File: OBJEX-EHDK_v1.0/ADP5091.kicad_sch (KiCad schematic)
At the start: 33 parts, among them J15 Solar, J16 Vout1, J17 Vout2, J18 Conn_01x02, J19 Conn_01x02, J20 TestPoint - Black, J21 TestPoint - Red, J22 TestPoint - Purple, J23 TestPoint - Orange, J24 TestPoint - Black, J25 TestPoint - Black, U2 ADP5091

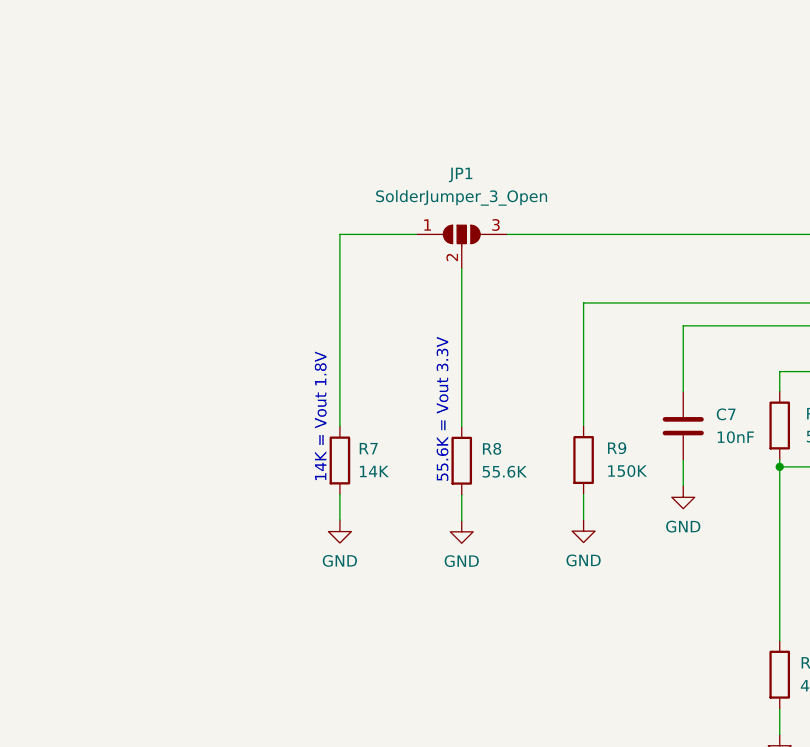
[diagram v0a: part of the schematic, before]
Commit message: SCH first review
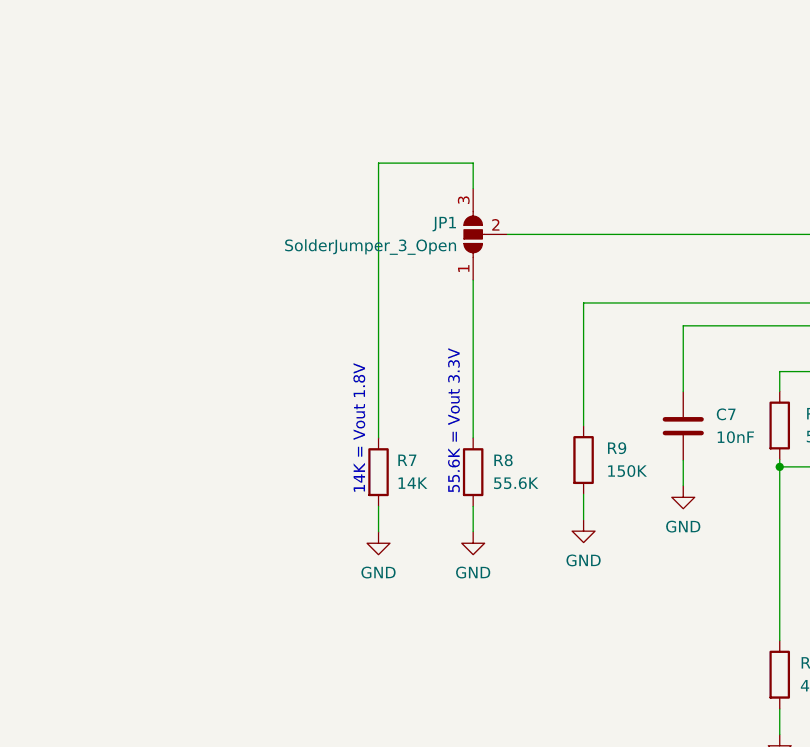
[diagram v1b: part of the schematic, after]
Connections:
- net at U2.20 (VID): now also JP1.2 (C); no longer JP1.3 (B)
- net at R8.1: now also JP1.1 (A); no longer JP1.2 (C)
- net at R7.1: now also JP1.3 (B); no longer JP1.1 (A)
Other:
- moved on the sheet: JP1, R7, R8
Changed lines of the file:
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@@
+    (stroke (width 0) (type default) (color 0 0 0 0))
+  )
+  (wire (pts (xy 69.0626 85.2678) (xy 69.0626 88.1126))
     (stroke (width 0) (type default) (color 0 0 0 0))
   )
@@
     (stroke (width 0) (type default) (color 0 0 0 0))
   )
+  (wire (pts (xy 58.547 85.2678) (xy 69.0626 85.2678))
+    (stroke (width 0) (type default) (color 0 0 0 0))
+  )
   (wire (pts (xy 137.6426 76.0222) (xy 137.6426 77.9526))
     (stroke (width 0) (type default) (color 0 0 0 0))
@@
     (stroke (width 0) (type default) (color 0 0 0 0))
   )
-  (wire (pts (xy 54.2544 93.1926) (xy 54.2544 114.5032))
+  (wire (pts (xy 58.547 85.2678) (xy 58.547 115.7986))
     (stroke (width 0) (type default) (color 0 0 0 0))
   )
@@
     (stroke (width 0) (type default) (color 0 0 0 0))
   )
-  (wire (pts (xy 67.7926 114.5286) (xy 67.7926 97.0026))
+  (wire (pts (xy 69.0626 115.7986) (xy 69.0626 98.2726))
     (stroke (width 0) (type default) (color 0 0 0 0))
   )
@@
     (stroke (width 0) (type default) (color 0 0 0 0))
   )
-  (wire (pts (xy 62.7126 93.1926) (xy 54.2544 93.1926))
-    (stroke (width 0) (type default) (color 0 0 0 0))
-  )
   (wire (pts (xy 212.217 103.3526) (xy 212.217 105.664))
     (stroke (width 0) (type default) (color 0 0 0 0))
@@
     (stroke (width 0) (type default) (color 0 0 0 0))
   )
-  (wire (pts (xy 54.2544 122.1232) (xy 54.2544 124.9426))
+  (wire (pts (xy 58.547 123.4186) (xy 58.547 126.238))
     (stroke (width 0) (type default) (color 0 0 0 0))
   )
@@
     (stroke (width 0) (type default) (color 0 0 0 0))
   )
-  (wire (pts (xy 67.7926 122.1486) (xy 67.7926 124.968))
+  (wire (pts (xy 69.0626 123.4186) (xy 69.0626 126.238))
     (stroke (width 0) (type default) (color 0 0 0 0))
   )
@@
     (effects (font (size 5 5) (thickness 0.8) bold) (justify left bottom))
   )
-  (text "55.6K = Vout 3.3V" (at 66.4464 120.9548 90)
+  (text "55.6K = Vout 3.3V" (at 67.7164 122.2248 90)
     (effects (font (size 1.27 1.27)) (justify left bottom))
   )
@@
     (effects (font (size 3.5 3.5) italic) (justify left bottom))
   )
-  (text "14K = Vout 1.8V" (at 52.9082 120.9294 90)
+  (text "14K = Vout 1.8V" (at 57.2008 122.2248 90)
     (effects (font (size 1.27 1.27)) (justify left bottom))
   )
@@
     (pin "2")
   )
-  (symbol (lib_id "power:GND") (at 54.2544 124.9426 0) (unit 1)
-    (in_bom yes) (on_board yes) (fields_autoplaced)
-    (property "Reference" "#PWR0125" (id 0) (at 54.2544 131.2926 0)
-      (effects (font (size 1.27 1.27)) hide)
-    )
-    (property "Value" "GND" (id 1) (at 54.2544 129.5146 0))
-    (property "Footprint" "" (id 2) (at 54.2544 124.9426 0)
-      (effects (font (size 1.27 1.27)) hide)
-    )
-    (property "Datasheet" "" (id 3) (at 54.2544 124.9426 0)
+  (symbol (lib_id "power:GND") (at 58.547 126.238 0) (unit 1)
+    (in_bom yes) (on_board yes) (fields_autoplaced)
+    (property "Reference" "#PWR0125" (id 0) (at 58.547 132.588 0)
+      (effects (font (size 1.27 1.27)) hide)
+    )
+    (property "Value" "GND" (id 1) (at 58.547 130.81 0))
+    (property "Footprint" "" (id 2) (at 58.547 126.238 0)
+      (effects (font (size 1.27 1.27)) hide)
+    )
+    (property "Datasheet" "" (id 3) (at 58.547 126.238 0)
       (effects (font (size 1.27 1.27)) hide)
     )
@@
     (pin "2")
   )
-  (symbol (lib_id "power:GND") (at 67.7926 124.968 0) (unit 1)
-    (in_bom yes) (on_board yes) (fields_autoplaced)
-    (property "Reference" "#PWR0124" (id 0) (at 67.7926 131.318 0)
-      (effects (font (size 1.27 1.27)) hide)
-    )
-    (property "Value" "GND" (id 1) (at 67.7926 129.54 0))
-    (property "Footprint" "" (id 2) (at 67.7926 124.968 0)
-      (effects (font (size 1.27 1.27)) hide)
-    )
-    (property "Datasheet" "" (id 3) (at 67.7926 124.968 0)
+  (symbol (lib_id "power:GND") (at 69.0626 126.238 0) (unit 1)
+    (in_bom yes) (on_board yes) (fields_autoplaced)
+    (property "Reference" "#PWR0124" (id 0) (at 69.0626 132.588 0)
+      (effects (font (size 1.27 1.27)) hide)
+    )
+    (property "Value" "GND" (id 1) (at 69.0626 130.81 0))
+    (property "Footprint" "" (id 2) (at 69.0626 126.238 0)
+      (effects (font (size 1.27 1.27)) hide)
+    )
+    (property "Datasheet" "" (id 3) (at 69.0626 126.238 0)
       (effects (font (size 1.27 1.27)) hide)
     )
@@
     (pin "1")
   )
-  (symbol (lib_id "Device:R") (at 67.7926 118.3386 0) (unit 1)
-    (in_bom yes) (on_board yes) (fields_autoplaced)
-    (property "Reference" "R8" (id 0) (at 69.977 117.0685 0)
-      (effects (font (size 1.27 1.27)) (justify left))
-    )
-    (property "Value" "55.6K" (id 1) (at 69.977 119.6085 0)
-      (effects (font (size 1.27 1.27)) (justify left))
-    )
-    (property "Footprint" "Resistor_SMD:R_0603_1608Metric" (id 2) (at 66.0146 118.3386 90)
-      (effects (font (size 1.27 1.27)) hide)
-    )
-    (property "Datasheet" "~" (id 3) (at 67.7926 118.3386 0)
+  (symbol (lib_id "Device:R") (at 69.0626 119.6086 0) (unit 1)
+    (in_bom yes) (on_board yes) (fields_autoplaced)
+    (property "Reference" "R8" (id 0) (at 71.247 118.3385 0)
+      (effects (font (size 1.27 1.27)) (justify left))
+    )
+    (property "Value" "55.6K" (id 1) (at 71.247 120.8785 0)
+      (effects (font (size 1.27 1.27)) (justify left))
+    )
+    (property "Footprint" "Resistor_SMD:R_0603_1608Metric" (id 2) (at 67.2846 119.6086 90)
+      (effects (font (size 1.27 1.27)) hide)
+    )
+    (property "Datasheet" "~" (id 3) (at 69.0626 119.6086 0)
       (effects (font (size 1.27 1.27)) hide)
     )
@@
     (pin "2")
   )
-  (symbol (lib_id "Jumper:SolderJumper_3_Open") (at 67.7926 93.1926 0) (unit 1)
-    (in_bom yes) (on_board yes) (fields_autoplaced)
-    (property "Reference" "JP1" (id 0) (at 67.7926 86.4616 0))
-    (property "Value" "SolderJumper_3_Open" (id 1) (at 67.7926 89.0016 0))
-    (property "Footprint" "Jumper:SolderJumper-3_P1.3mm_Open_Pad1.0x1.5mm_NumberLabels" (id 2) (at 67.7926 93.1926 0)
-      (effects (font (size 1.27 1.27)) hide)
-    )
-    (property "Datasheet" "~" (id 3) (at 67.7926 93.1926 0)
+  (symbol (lib_id "Jumper:SolderJumper_3_Open") (at 69.0626 93.1926 90) (unit 1)
+    (in_bom yes) (on_board yes) (fields_autoplaced)
+    (property "Reference" "JP1" (id 0) (at 67.31 91.9225 90)
+      (effects (font (size 1.27 1.27)) (justify left))
+    )
+    (property "Value" "SolderJumper_3_Open" (id 1) (at 67.31 94.4625 90)
+      (effects (font (size 1.27 1.27)) (justify left))
+    )
+    (property "Footprint" "Jumper:SolderJumper-3_P1.3mm_Open_Pad1.0x1.5mm_NumberLabels" (id 2) (at 69.0626 93.1926 0)
+      (effects (font (size 1.27 1.27)) hide)
+    )
+    (property "Datasheet" "~" (id 3) (at 69.0626 93.1926 0)
       (effects (font (size 1.27 1.27)) hide)
     )
@@
     (pin "2")
   )
-  (symbol (lib_id "Device:R") (at 54.2544 118.3132 0) (unit 1)
-    (in_bom yes) (on_board yes) (fields_autoplaced)
-    (property "Reference" "R7" (id 0) (at 56.2864 117.0431 0)
-      (effects (font (size 1.27 1.27)) (justify left))
-    )
-    (property "Value" "14K" (id 1) (at 56.2864 119.5831 0)
-      (effects (font (size 1.27 1.27)) (justify left))
-    )
-    (property "Footprint" "Resistor_SMD:R_0603_1608Metric" (id 2) (at 52.4764 118.3132 90)
-      (effects (font (size 1.27 1.27)) hide)
-    )
-    (property "Datasheet" "~" (id 3) (at 54.2544 118.3132 0)
-      (effects (font (size 1.27 1.27)) hide)
-    )
+  (symbol (lib_id "Device:R") (at 58.547 119.6086 0) (unit 1)
+    (in_bom yes) (on_board yes) (fields_autoplaced)
+    (property "Reference" "R7" (id 0) (at 60.579 118.3385 0)
+      (effects (font (size 1.27 1.27)) (justify left))
+    )
+    (property "Value" "14K" (id 1) (at 60.579 120.8785 0)
+      (effects (font (size 1.27 1.27)) (justify left))
+    )
+    (property "Footprint" "Resistor_SMD:R_0603_1608Metric" (id 2) (at 56.769 119.6086 90)
+      (effects (font (size 1.27 1.27)) hide)
+    )
+    (property "Datasheet" "~" (id 3) (at 58.547 119.6086 0)
+      (effects (font (size 1.27 1.27)) hide)
+    )
